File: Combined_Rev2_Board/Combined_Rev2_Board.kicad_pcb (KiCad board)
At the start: 4 copper layers, 121.9 x 106.8 mm, 178 parts, among them CN1 Conn_02x19_Odd_Even, CN1 USB_C_Receptacle_PowerOnly_6P, CN2 B2B-XH-A, CN2 Conn_02x19_Odd_Even, CN3 522070860, CN3 Molex FPC 541044031, CN4 Conn_01x02_Pin, CN4 Molex FPC 52271-0679, CN5 Conn_01x02_Pin, CN5 Conn_02x20_Odd_Even, CN6 Conn_01x02_Pin, CN7 Conn_01x02_Pin, J1 522070860, J1 Conn_01x02_Pin, J1 MIllMaxSpringConnector, J2 MIllMaxSpringConnector, J3 MIllMaxSpringConnector, J4 MIllMaxSpringConnector, J5 Conn_01x02_Pin, J5 MIllMaxSpringConnector, J6 Conn_01x02_Pin, J6 MIllMaxSpringConnector, J7 Conn_01x02_Pin, J7 MIllMaxSpringConnector, J8 MIllMaxSpringConnector, Q1 SI2347DS-TI-GE3CT, Q3 DMG3406L-7, Q4 SSM3J358R, SW2 Rocker Switch SPST, U1 AP5725WG-7, U10 LTC6252, U11 ADA4807-1, U11 MCP73831-2-OT, U12 LTC6252, U13 ADA4807-1, U14 LTC6252, U15 ADA4807-1, U16 LTC6252, U17 ADA4807-1, U2 ADA4807-2ACP, U2 LD39200, U3 ADR4530, U4 ADA4807-2ACP, U5 ADP7118-1.8, U6 ADA4807-2ACP, U7 AD4002_LFSCP-10, U8 AD4002_LFSCP-10, U8 TPS2400, U9 LD39200_Fixed

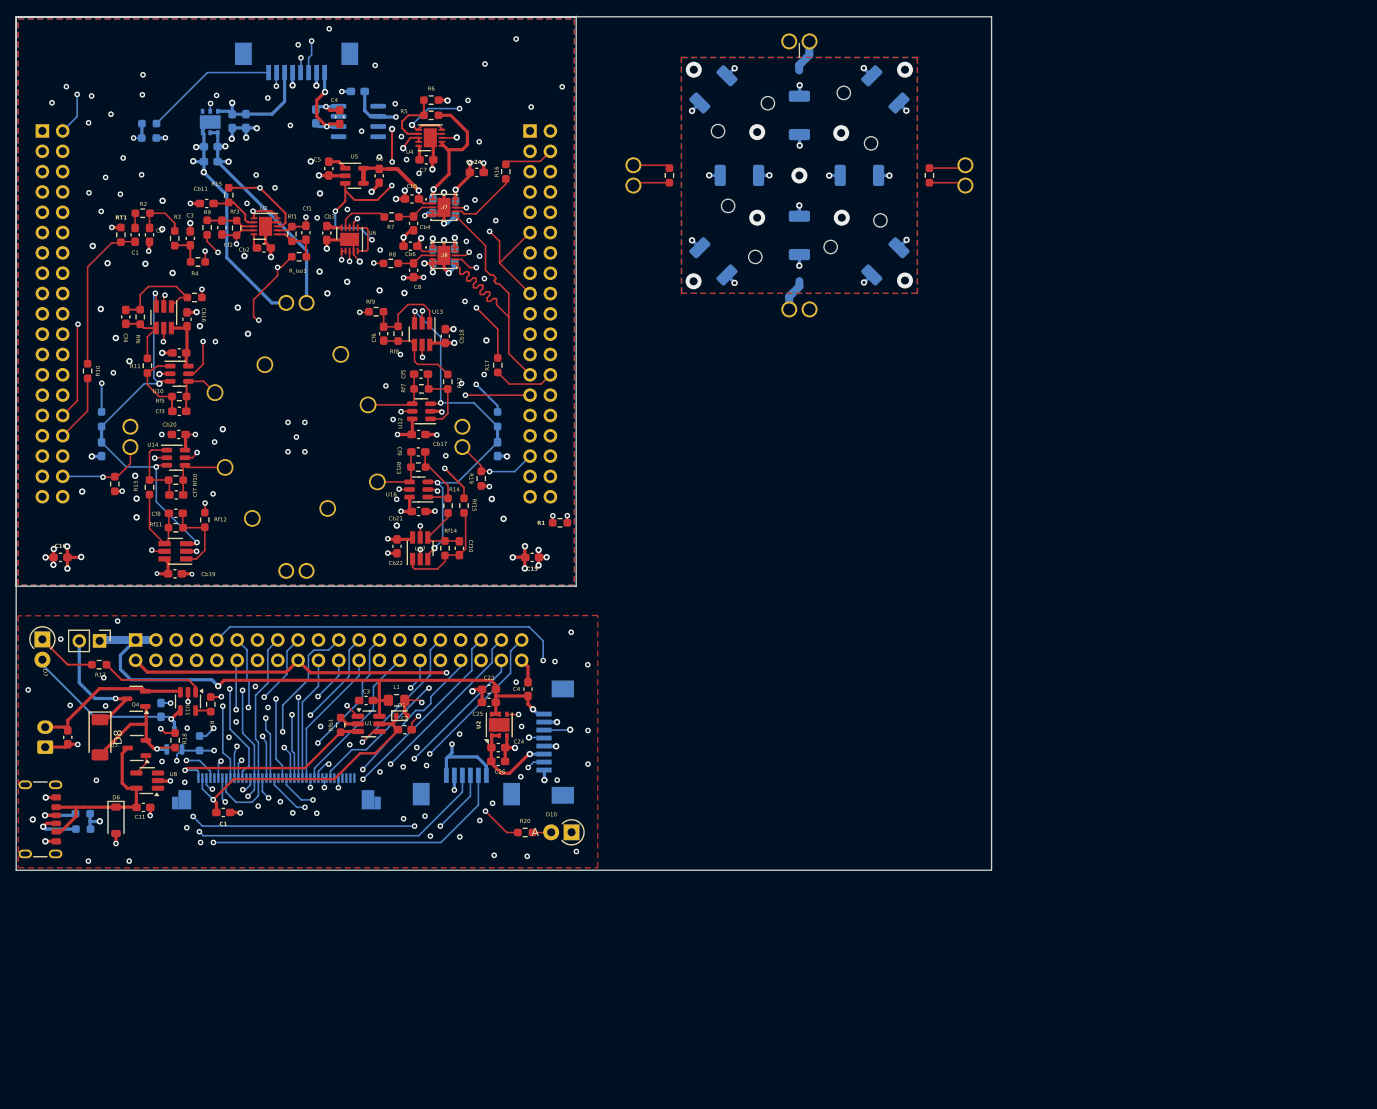
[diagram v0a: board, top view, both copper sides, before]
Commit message: Final commit before order
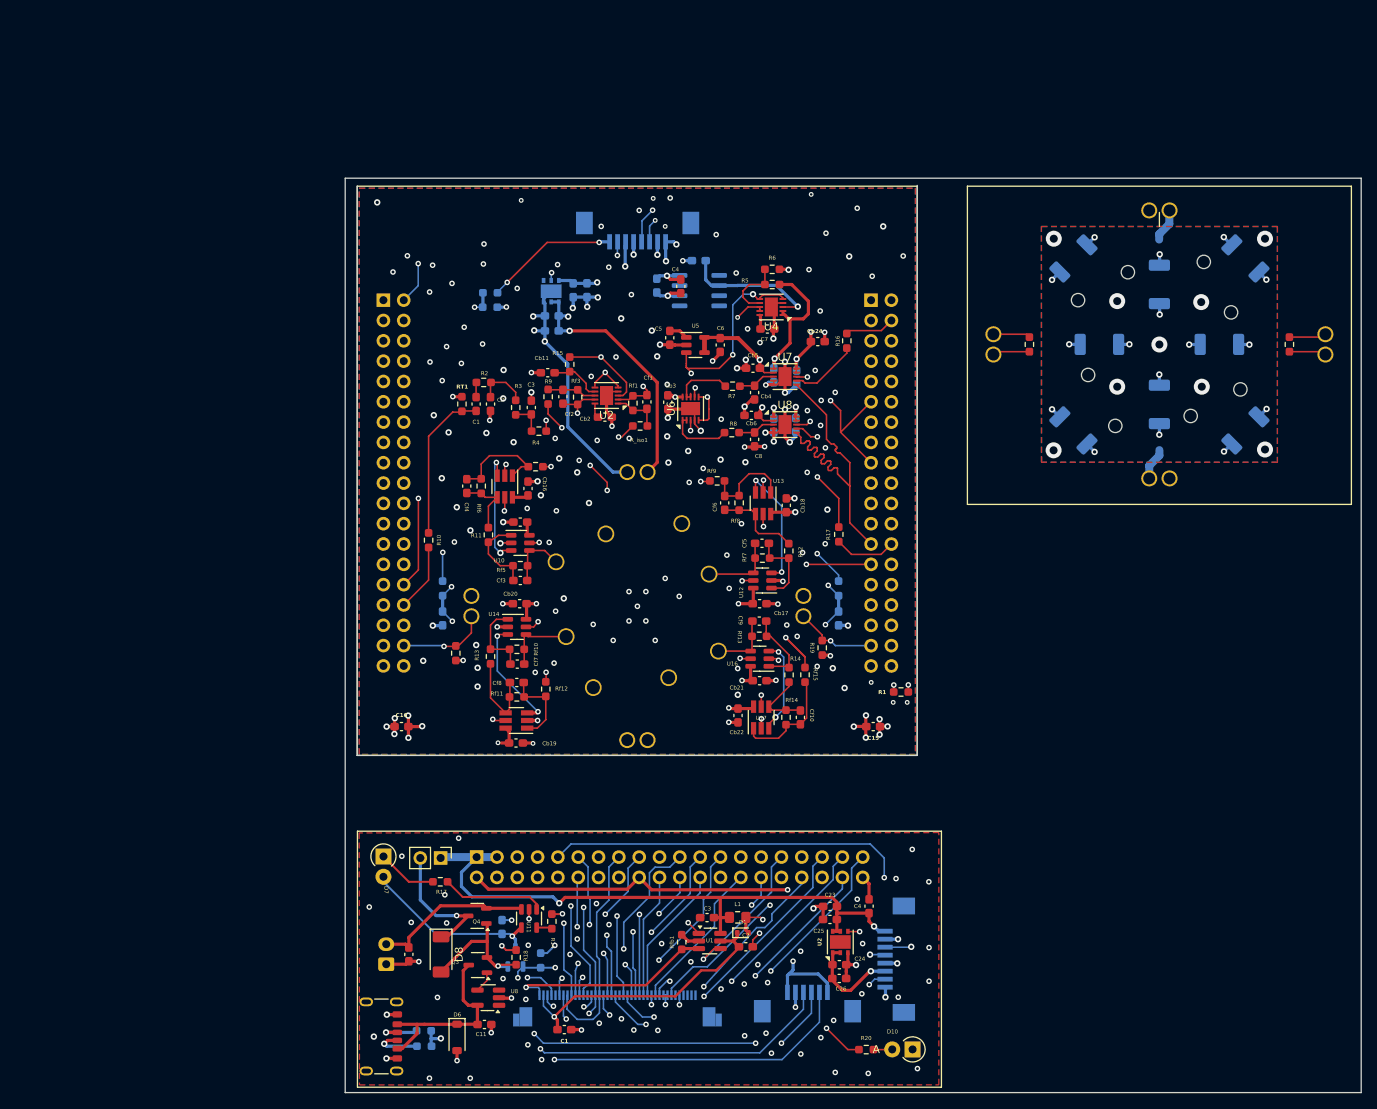
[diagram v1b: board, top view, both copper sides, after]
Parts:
- removed the C1 at (32.8, 109.3)
- removed the C1 at (21.7, 37.1)
- removed the C11 at (22.8, 108.7)
- removed the C11 at (49.6, 19.2)
- removed the C2 at (23.5, 37.1)
- removed the C2 at (55.5, 98.9)
- removed the C3 at (28.6, 37.5)
- removed the C3 at (50.6, 95.3)
- removed the C4 at (47.3, 22.4)
- removed the C4 at (70.9, 93.9)
- removed the CN1 at (8.80, 110.1)
- removed the CN1 at (10.2, 24.1)
- removed the CN2 at (71.1, 24.1)
- removed the CN2 at (10.5, 101.1)
- removed the CN3 at (39.4, 107.5)
- removed the CN3 at (41.9, 13.7)
- removed the CN4 at (21.1, 62.3)
- removed the CN4 at (63.2, 108.1)
- removed the CN5 at (62.6, 62.3)
- removed the CN5 at (21.8, 87.7)
- removed the J1 at (51.9, 66.6)
- removed the J1 at (104.8, 12.9)
- removed the J1 at (76.0, 100.5)
- removed the J5 at (51.5, 57.0)
- removed the J5 at (104.8, 46.4)
- removed the J6 at (84.0, 29.6)
- removed the J6 at (32.7, 55.0)
- removed the J7 at (47.5, 52.0)
- removed the J7 at (125.5, 29.6)
- removed the R1 at (74.8, 73.1)
- removed the R1 at (15.2, 109.4)
- removed the R10 at (15.8, 54.1)
- removed the R10 at (104.8, 22.1)
- removed the R11 at (23.3, 53.4)
- removed the R11 at (94.0, 18.9)
- removed the R12 at (60.8, 55.4)
- removed the R12 at (97.3, 29.6)
- removed the R13 at (23.5, 68.6)
- removed the R13 at (112.3, 29.6)
- removed the R14 at (60.9, 70.9)
- removed the R14 at (31.2, 95.8)
- removed the R14 at (104.8, 37.1)
- removed the R15 at (33.4, 32.1)
- removed the R15 at (94.0, 40.4)
- removed the R16 at (68.1, 29.2)
- removed the R16 at (115.5, 40.4)
- removed the R17 at (67.1, 53.4)
- removed the R17 at (17.3, 90.8)
- removed the R18 at (19.2, 68.2)
- removed the R18 at (26.7, 100.3)
- removed the R2 at (22.7, 34.4)
- removed the R2 at (15.3, 111.4)
- removed the R20 at (70.5, 111.8)
- removed the R20 at (23.5, 23.2)
- removed the R9 at (30.7, 36.2)
- removed the R9 at (115.5, 18.9)
- removed the U11 at (25.3, 47.4)
- removed the U11 at (28.4, 95.4)
- removed the U2 at (67.3, 98.3)
- removed the U2 at (38.0, 36.0)
- removed the U8 at (23.3, 105.3)
- removed the U8 at (60.4, 39.6)
- added C1: 1uF, Capacitor_SMD:C_0603_1608Metric_Pad1.08x0.95mm_HandSolder, F.Cu at (75.4, 136.4)
- added C1: 100p, Capacitor_SMD:C_0603_1608Metric_Pad1.08x0.95mm_HandSolder, F.Cu at (64.4, 58.2)
- added C11: 0.1u, Capacitor_SMD:C_0603_1608Metric_Pad1.08x0.95mm_HandSolder, F.Cu at (65.4, 135.8)
- added C11: 1uF, Capacitor_SMD:C_0603_1608Metric_Pad1.08x0.95mm_HandSolder, B.Cu at (92.2, 40.3)
- added C2: 1uF, Capacitor_SMD:C_0603_1608Metric_Pad1.08x0.95mm_HandSolder, F.Cu at (98.1, 126.1)
- added C2: 47p, Capacitor_SMD:C_0603_1608Metric_Pad1.08x0.95mm_HandSolder, F.Cu at (66.2, 58.2)
- added C3: 1uF, Capacitor_SMD:C_0603_1608Metric_Pad1.08x0.95mm_HandSolder, F.Cu at (93.2, 122.4)
- added C3: 47p, Capacitor_SMD:C_0603_1608Metric_Pad1.08x0.95mm_HandSolder, F.Cu at (71.3, 58.7)
- added C4: 1uF, Capacitor_SMD:C_0603_1608Metric_Pad1.08x0.95mm_HandSolder, F.Cu at (90.0, 43.5)
- added C4: 22u, Capacitor_SMD:C_0603_1608Metric_Pad1.08x0.95mm_HandSolder, F.Cu at (113.5, 121.0)
- added CN1: USB_C_Receptacle_PowerOnly_6P, Connector_USB:USB_C_Receptacle_GCT_USB4125-xx-x_6P_TopMnt_Horizontal, F.Cu at (51.4, 137.3)
- added CN1: Conn_02x19_Odd_Even, Connector_PinSocket_2.54mm:PinSocket_2x19_P2.54mm_Vertical, B.Cu at (52.8, 45.2)
- added CN2: Conn_02x19_Odd_Even, Connector_PinSocket_2.54mm:PinSocket_2x19_P2.54mm_Vertical, B.Cu at (113.7, 45.2)
- added CN2: B2B-XH-A, Connector_JST:JST_XH_B2B-XH-A_1x02_P2.50mm_Vertical, B.Cu at (53.1, 128.2)
- added CN3: 522070860, GenIILibrary:CON_522070860_MOL, B.Cu at (84.5, 34.8)
- added CN3: Molex FPC 541044031, GenIILibrary:CON_541044031_MOL, B.Cu at (82.0, 134.6)
- added CN4: Conn_01x02_Pin, GenIILibrary:Samtec_Pin_Socket_SS_102_G_2, F.Cu at (63.8, 83.5)
- added CN4: Molex FPC 52271-0679, GenIILibrary:MOLEX_52271-0679, B.Cu at (105.8, 135.3)
- added CN5: Conn_01x02_Pin, GenIILibrary:Samtec_Pin_Socket_SS_102_G_2, F.Cu at (105.3, 83.5)
- added CN5: Conn_02x20_Odd_Even, Connector_PinHeader_2.54mm:PinHeader_2x20_P2.54mm_Vertical, B.Cu at (64.4, 114.9)
- added J1: MIllMaxSpringConnector, TCGenI_Rev3_Redo:MillMax_0914-2, F.Cu at (94.5, 87.8)
- added J1: Conn_01x02_Pin, GenIILibrary:Samtec_Pin_Socket_SS_102_G_2, F.Cu at (149.8, 34.0)
- added J1: 522070860, GenIILibrary:CON_522070860_MOL, B.Cu at (118.6, 127.6)
- added J5: MIllMaxSpringConnector, TCGenI_Rev3_Redo:MillMax_0914-2, F.Cu at (94.1, 78.1)
- added J5: Conn_01x02_Pin, GenIILibrary:Samtec_Pin_Socket_SS_102_G_2, F.Cu at (149.8, 67.5)
- added J6: Conn_01x02_Pin, GenIILibrary:Samtec_Pin_Socket_SS_102_G_2, F.Cu at (129.0, 50.8)
- added J6: MIllMaxSpringConnector, TCGenI_Rev3_Redo:MillMax_0914-2, F.Cu at (75.3, 76.1)
- added J7: MIllMaxSpringConnector, TCGenI_Rev3_Redo:MillMax_0914-2, F.Cu at (90.1, 73.2)
- added J7: Conn_01x02_Pin, GenIILibrary:Samtec_Pin_Socket_SS_102_G_2, F.Cu at (170.5, 50.8)
- added R1: 33, Resistor_SMD:R_0603_1608Metric_Pad0.98x0.95mm_HandSolder, F.Cu at (117.5, 94.2)
- added R1: 5.1k, Resistor_SMD:R_0603_1608Metric_Pad0.98x0.95mm_HandSolder, B.Cu at (57.8, 136.6)
- added R10: 33, Resistor_SMD:R_0603_1608Metric_Pad0.98x0.95mm_HandSolder, F.Cu at (58.4, 75.2)
- added R10: 50, Resistor_SMD:R_2010_5025Metric_Pad1.40x2.65mm_HandSolder, B.Cu at (149.8, 43.3)
- added R11: 1k, Resistor_SMD:R_0603_1608Metric_Pad0.98x0.95mm_HandSolder, F.Cu at (65.9, 74.6)
- added R11: 50, Resistor_SMD:R_2010_5025Metric_Pad1.40x2.65mm_HandSolder, B.Cu at (139.0, 40.0)
- added R12: 1k, Resistor_SMD:R_0603_1608Metric_Pad0.98x0.95mm_HandSolder, F.Cu at (103.5, 76.6)
- added R12: 50, Resistor_SMD:R_2010_5025Metric_Pad1.40x2.65mm_HandSolder, B.Cu at (142.3, 50.8)
- added R13: 1k, Resistor_SMD:R_0603_1608Metric_Pad0.98x0.95mm_HandSolder, F.Cu at (66.2, 89.8)
- added R13: 50, Resistor_SMD:R_2010_5025Metric_Pad1.40x2.65mm_HandSolder, B.Cu at (157.3, 50.8)
- added R14: 1k, Resistor_SMD:R_0603_1608Metric_Pad0.98x0.95mm_HandSolder, F.Cu at (103.5, 92.1)
- added R14: 2k, Resistor_SMD:R_0603_1608Metric_Pad0.98x0.95mm_HandSolder, F.Cu at (73.8, 122.9)
- added R14: 50, Resistor_SMD:R_2010_5025Metric_Pad1.40x2.65mm_HandSolder, B.Cu at (149.8, 58.3)
- added R15: 1k, Resistor_SMD:R_0603_1608Metric_Pad0.98x0.95mm_HandSolder, F.Cu at (76.1, 53.3)
- added R15: 50, Resistor_SMD:R_2010_5025Metric_Pad1.40x2.65mm_HandSolder, B.Cu at (139.0, 61.5)
- added R16: 33, Resistor_SMD:R_0603_1608Metric_Pad0.98x0.95mm_HandSolder, F.Cu at (110.7, 50.3)
- added R16: 50, Resistor_SMD:R_2010_5025Metric_Pad1.40x2.65mm_HandSolder, B.Cu at (160.5, 61.5)
- added R17: 1k, Resistor_SMD:R_0603_1608Metric_Pad0.98x0.95mm_HandSolder, F.Cu at (59.9, 118.0)
- added R17: 33, Resistor_SMD:R_0603_1608Metric_Pad0.98x0.95mm_HandSolder, F.Cu at (109.7, 74.5)
- added R18: 1k, Resistor_SMD:R_0603_1608Metric_Pad0.98x0.95mm_HandSolder, F.Cu at (61.8, 89.4)
- added R18: 10k, Resistor_SMD:R_0603_1608Metric_Pad0.98x0.95mm_HandSolder, F.Cu at (69.4, 127.4)
- added R2: 10k, Resistor_SMD:R_0603_1608Metric_Pad0.98x0.95mm_HandSolder, F.Cu at (65.3, 55.5)
- added R2: 5.1k, Resistor_SMD:R_0603_1608Metric_Pad0.98x0.95mm_HandSolder, B.Cu at (57.9, 138.5)
- added R20: 1k, Resistor_SMD:R_0603_1608Metric_Pad0.98x0.95mm_HandSolder, F.Cu at (113.1, 138.9)
- added R20: 10k, Resistor_SMD:R_0603_1608Metric_Pad0.98x0.95mm_HandSolder, B.Cu at (66.1, 44.3)
- added R9: 1k, Resistor_SMD:R_0603_1608Metric_Pad0.98x0.95mm_HandSolder, F.Cu at (73.4, 57.3)
- added R9: 50, Resistor_SMD:R_2010_5025Metric_Pad1.40x2.65mm_HandSolder, B.Cu at (160.5, 40.0)
- added U11: MCP73831-2-OT, Package_TO_SOT_SMD:SOT-23-5, F.Cu at (71.0, 122.5)
- added U11: ADA4807-1, Package_TO_SOT_SMD:SOT-23-6_Handsoldering, F.Cu at (68.0, 68.5)
- added U2: LD39200, Package_DFN_QFN:DFN-6-1EP_3x3mm_P0.95mm_EP1.7x2.6mm, F.Cu at (109.9, 125.5)
- added U2: ADA4807-2ACP, CustomPaste:LFCSP-WD-10-1EP_3x3mm_P0.5mm_EP1.64x2.38mm, F.Cu at (80.7, 57.2)
- added U8: TPS2400, Package_TO_SOT_SMD:SOT-23-5_HandSoldering, F.Cu at (65.9, 132.4)
- added U8: AD4002_LFSCP-10, Package_CSP:LFCSP-WD-10-1EP_3x3mm_P0.5mm_EP1.64x2.38mm, F.Cu at (103.0, 60.8)
- RT1: value 0 -> NC
- U4, U6: footprint Package_CSP:LFCSP-WD-10-1EP_3x3mm_P0.5mm_EP1.64x2.38mm -> CustomPaste:LFCSP-WD-10-1EP_3x3mm_P0.5mm_EP1.64x2.38mm
- U7: footprint footprints:CP_10_9_ADI -> Package_CSP:LFCSP-WD-10-1EP_3x3mm_P0.5mm_EP1.64x2.38mm
- moved C20 50.5 mm to (56.0, 127.0)
- moved C23 50.5 mm to (108.6, 121.0)
- moved C25 50.5 mm to (108.6, 122.7)
- moved D1 50.5 mm to (97.7, 124.3)
- moved D10 50.5 mm to (118.9, 138.9)
- moved D6 50.5 mm to (62.0, 137.4)
- moved D8 50.5 mm to (60.0, 127.0)
- moved Q1 50.5 mm to (69.3, 127.4)
- moved Q3 50.5 mm to (64.6, 128.4)
- moved RPU1 50.5 mm to (72.4, 127.8)
- moved Rfb1 50.5 mm to (90.1, 125.5)
- moved C19 50.5 mm to (67.6, 123.6)
- moved D7 50.5 mm to (52.8, 114.8)
- moved L1 50.5 mm to (97.1, 122.4)
- moved Q4 50.5 mm to (64.5, 122.2)
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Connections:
- C10 pad 1: (no net) -> GND
- C10 pad 2: (no net) -> Vdd_Main
- C12 pad 1: (no net) -> /Heater_Interface/Heater+
- C12 pad 2: (no net) -> GND
- C13 pad 1: (no net) -> Vcc
- C13 pad 2: (no net) -> GND
- C14 pad 1: (no net) -> /Heater_Interface/Heater+
- C14 pad 2: (no net) -> GND
- C15 pad 1: (no net) -> GND
- C15 pad 2: (no net) -> Vdd_Main
- C16 pad 1: (no net) -> GND
- C16 pad 2: (no net) -> Vdd_Main
- C19 pad 1: (no net) -> GND
- C19 pad 2: (no net) -> Net-(D7-A)
- C20 pad 1: (no net) -> /V_Batt
- C20 pad 2: (no net) -> GND
- C23 pad 1: (no net) -> GND
- C23 pad 2: (no net) -> /Vcc
- C24 pad 1: (no net) -> /3V3_Main
- C24 pad 2: (no net) -> GND
- C25 pad 1: (no net) -> /Vcc
- C25 pad 2: (no net) -> GND
- C26 pad 1: (no net) -> /3V3_Main
- C26 pad 2: (no net) -> GND
- C5 pad 1: (no net) -> Vdd_Main
- C5 pad 2: (no net) -> GND
- C6 pad 1: (no net) -> Vdd_ADC
- C6 pad 2: (no net) -> GND
- C7 pad 1: (no net) -> Vdd_Main
- C7 pad 2: (no net) -> GND
- C8 pad 1: (no net) -> GND
- C8 pad 2: (no net) -> Net-(U8-IN+)
- C9 pad 1: (no net) -> GND
- C9 pad 2: (no net) -> Vcc
- CN6 pad 1: (no net) -> unconnected-(CN6-Pin_1-Pad1)
- CN6 pad 2: (no net) -> unconnected-(CN6-Pin_2-Pad2)
- CN7 pad 1: (no net) -> GND
- CN7 pad 2: (no net) -> /Heater_Interface/Heater+
- Cb1 pad 1: (no net) -> GND
- Cb1 pad 2: (no net) -> /ABBCore_Alt/TIA_2/V_MID
- Cb10 pad 1: (no net) -> GND
- Cb10 pad 2: (no net) -> Vdd_Main
- Cb11 pad 1: (no net) -> GND
- Cb11 pad 2: (no net) -> Net-(U2B-+)
- Cb12 pad 1: (no net) -> GND
- Cb12 pad 2: (no net) -> /ABBCore_Alt/TIA_1/V_MID
- Cb15 pad 1: (no net) -> GND
- Cb15 pad 2: (no net) -> Vdd_Main
- Cb16 pad 1: (no net) -> GND
- Cb16 pad 2: (no net) -> Vdd_Main
- Cb17 pad 1: (no net) -> GND
- Cb17 pad 2: (no net) -> Vdd_Main
- Cb18 pad 1: (no net) -> GND
- Cb18 pad 2: (no net) -> Vdd_Main
- Cb19 pad 1: (no net) -> GND
- Cb19 pad 2: (no net) -> Vdd_Main
- Cb2 pad 1: (no net) -> GND
- Cb2 pad 2: (no net) -> Vdd_Main
- Cb20 pad 1: (no net) -> GND
- Cb20 pad 2: (no net) -> Vdd_Main
- Cb21 pad 1: (no net) -> GND
- Cb21 pad 2: (no net) -> Vdd_Main
- Cb22 pad 1: (no net) -> GND
- Cb22 pad 2: (no net) -> Vdd_Main
- Cb24 pad 1: (no net) -> GND
- Cb24 pad 2: (no net) -> Vdd_Main
- Cb3 pad 1: (no net) -> Vdd_Main
- Cb3 pad 2: (no net) -> GND
- Cb4 pad 1: (no net) -> GND
- Cb4 pad 2: (no net) -> Net-(U7-IN+)
- Cb5 pad 1: (no net) -> Vdd_ADC
- Cb5 pad 2: (no net) -> GND
- Cb6 pad 1: (no net) -> Vdd_ADC
- Cb6 pad 2: (no net) -> GND
- Cb7 pad 1: (no net) -> GND
- Cb7 pad 2: (no net) -> ADC_VREF
- Cb8 pad 1: (no net) -> GND
- Cb8 pad 2: (no net) -> ADC_VREF
- Cb9 pad 1: (no net) -> GND
- Cb9 pad 2: (no net) -> Vdd_Main
- Cf1 pad 1: (no net) -> Net-(Cf1-Pad1)
- Cf1 pad 2: (no net) -> Net-(U2A--)
- Cf10 pad 1: (no net) -> Net-(U17--)
- Cf10 pad 2: (no net) -> Net-(Cf10-Pad2)
- Cf2 pad 1: (no net) -> Net-(U2B--)
- Cf2 pad 2: (no net) -> /ABBCore_Alt/V_Exc
- Cf3 pad 1: (no net) -> CCOut_1
- Cf3 pad 2: (no net) -> Net-(Cf3-Pad2)
- Cf4 pad 1: (no net) -> Net-(U11--)
- Cf4 pad 2: (no net) -> Net-(Cf4-Pad2)
- Cf5 pad 1: (no net) -> CCOut_2
- Cf5 pad 2: (no net) -> Net-(Cf5-Pad2)
- Cf6 pad 1: (no net) -> Net-(U13--)
- Cf6 pad 2: (no net) -> Net-(Cf6-Pad2)
- Cf7 pad 1: (no net) -> CCOut_3
- Cf7 pad 2: (no net) -> Net-(Cf7-Pad2)
- Cf8 pad 1: (no net) -> Net-(U15--)
- Cf8 pad 2: (no net) -> Net-(Cf8-Pad2)
- Cf9 pad 1: (no net) -> CCOut_4
- Cf9 pad 2: (no net) -> Net-(Cf9-Pad2)
- D1 pad 1: (no net) -> /LED+
- D1 pad 2: (no net) -> Net-(D1-A)
- D10 pad 1: (no net) -> GND
- D10 pad 2: (no net) -> Net-(D10-A)
- D6 pad 1: (no net) -> /Power_Management_Minimal/VBus
- D6 pad 2: (no net) -> GND
- D7 pad 1: (no net) -> Net-(D7-K)
- D7 pad 2: (no net) -> Net-(D7-A)
- D8 pad 1: (no net) -> Net-(D8-K)
- D8 pad 2: (no net) -> /Power_Management_Minimal/5V_USB
- J2 pad 1: (no net) -> CCOut_3
- J3 pad 1: (no net) -> /ABBCore_Alt/V_Drive
- J4 pad 1: (no net) -> /ABBCore_Alt/V_Drive
- J8 pad 1: (no net) -> /ABBCore_Alt/V_Drive
- L1 pad 1: (no net) -> /Vcc
- L1 pad 2: (no net) -> Net-(D1-A)
- Q1 pad 1: (no net) -> /~{CHARGE_EN}
- Q1 pad 2: (no net) -> /Power_Management_Minimal/5V_USB
- Q1 pad 3: (no net) -> Net-(D7-A)
- Q3 pad 1: (no net) -> Net-(Q3-G)
- Q3 pad 2: (no net) -> /Power_Management_Minimal/5V_USB
- Q3 pad 3: (no net) -> /Power_Management_Minimal/VBus
- Q4 pad 1: (no net) -> /Power_Management_Minimal/5V_USB
- Q4 pad 2: (no net) -> /V_Batt
- Q4 pad 3: (no net) -> Net-(D8-K)
- R19 pad 1: (no net) -> GND
- R19 pad 2: (no net) -> Vth_2
- R21 pad 1: (no net) -> /MCU Connections/PC1
- R21 pad 2: (no net) -> GND
- R3 pad 1: (no net) -> Net-(C2-Pad1)
- R3 pad 2: (no net) -> Net-(C3-Pad1)
- R4 pad 1: (no net) -> Net-(C3-Pad1)
- R4 pad 2: (no net) -> Net-(U2A--)
- R5 pad 1: (no net) -> ADC_VREF
- R5 pad 2: (no net) -> Net-(U4B-+)
- R6 pad 1: (no net) -> Net-(U4B-+)
- R6 pad 2: (no net) -> GND
- R7 pad 1: (no net) -> Net-(U7-IN+)
- R7 pad 2: (no net) -> Net-(U6B--)
- R8 pad 1: (no net) -> Net-(U8-IN+)
- R8 pad 2: (no net) -> Net-(U6A--)
- RPU1 pad 1: (no net) -> /~{CHARGE_EN}
- RPU1 pad 2: (no net) -> GND
- RT1 pad 1: (no net) -> GND
- RT1 pad 2: (no net) -> V_SIG
- R_iso1 pad 1: (no net) -> Net-(Cf1-Pad1)
- R_iso1 pad 2: (no net) -> /ABBCore_Alt/V_Drive
- Rf1 pad 1: (no net) -> Net-(Cf1-Pad1)
- Rf1 pad 2: (no net) -> Net-(U2A--)
- Rf10 pad 1: (no net) -> CCOut_3
- Rf10 pad 2: (no net) -> Net-(Cf7-Pad2)
- Rf11 pad 1: (no net) -> Net-(U15--)
- Rf11 pad 2: (no net) -> Net-(Cf8-Pad2)
- Rf12 pad 1: (no net) -> Net-(Cf8-Pad2)
- Rf12 pad 2: (no net) -> /ABBCore_Alt/V_Resp
- Rf13 pad 1: (no net) -> CCOut_4
- Rf13 pad 2: (no net) -> Net-(Cf9-Pad2)
- Rf14 pad 1: (no net) -> Net-(U17--)
- Rf14 pad 2: (no net) -> Net-(Cf10-Pad2)
- Rf15 pad 1: (no net) -> Net-(Cf10-Pad2)
- Rf15 pad 2: (no net) -> /ABBCore_Alt/V_Resp
- Rf16 pad 1: (no net) -> V_MID
- Rf16 pad 2: (no net) -> /ABBCore_Alt/TIA_2/V_MID
- Rf3 pad 1: (no net) -> Net-(U2B--)
- Rf3 pad 2: (no net) -> /ABBCore_Alt/V_Exc
- Rf4 pad 1: (no net) -> V_MID
- Rf4 pad 2: (no net) -> /ABBCore_Alt/TIA_1/V_MID
- Rf5 pad 1: (no net) -> CCOut_1
- Rf5 pad 2: (no net) -> Net-(Cf3-Pad2)
- Rf6 pad 1: (no net) -> Net-(U11--)
- Rf6 pad 2: (no net) -> Net-(Cf4-Pad2)
- Rf7 pad 1: (no net) -> CCOut_2
- Rf7 pad 2: (no net) -> Net-(Cf5-Pad2)
- Rf8 pad 1: (no net) -> Net-(U13--)
- Rf8 pad 2: (no net) -> Net-(Cf6-Pad2)
- Rf9 pad 1: (no net) -> Net-(Cf6-Pad2)
- Rf9 pad 2: (no net) -> /ABBCore_Alt/V_Resp
- Rfb1 pad 1: (no net) -> GND
- Rfb1 pad 2: (no net) -> /LED-
- Riso1 pad 1: (no net) -> Net-(Cf4-Pad2)
- Riso1 pad 2: (no net) -> /ABBCore_Alt/V_Resp
- SW2 pad 1: (no net) -> /Vcc
- SW2 pad 2: (no net) -> Net-(D8-K)
- TH5 pad 1: (no net) -> Net-(J7-Pin_1)
- TH5 pad 2: (no net) -> Net-(J7-Pin_2)
- TH7 pad 1: (no net) -> Net-(J6-Pin_1)
- TH7 pad 2: (no net) -> Net-(J6-Pin_2)
- U1 pad 1: (no net) -> Net-(D1-A)
- U1 pad 2: (no net) -> GND
- U1 pad 3: (no net) -> /LED-
- U1 pad 4: (no net) -> /PWM_EN
- U1 pad 5: (no net) -> /LED+
- U1 pad 6: (no net) -> /Vcc
- U10 pad 1: (no net) -> Net-(Cf3-Pad2)
- U10 pad 2: (no net) -> GND
- U10 pad 3: (no net) -> /ABBCore_Alt/TIA_1/V_MID
- U10 pad 4: (no net) -> CCOut_1
- U10 pad 5: (no net) -> ~{TIA1_SHDN}
- U10 pad 6: (no net) -> Vdd_Main
- U12 pad 1: (no net) -> Net-(Cf5-Pad2)
- U12 pad 2: (no net) -> GND
- U12 pad 3: (no net) -> /ABBCore_Alt/TIA_2/V_MID
- U12 pad 4: (no net) -> CCOut_2
- U12 pad 5: (no net) -> ~{TIA2_SHDN}
- U12 pad 6: (no net) -> Vdd_Main
- U13 pad 1: (no net) -> Net-(Cf6-Pad2)
- U13 pad 2: (no net) -> GND
- U13 pad 3: (no net) -> /ABBCore_Alt/TIA_2/V_MID
- U13 pad 4: (no net) -> Net-(U13--)
- U13 pad 5: (no net) -> ~{TIA2_SHDN}
- U13 pad 6: (no net) -> Vdd_Main
- U14 pad 1: (no net) -> Net-(Cf7-Pad2)
- U14 pad 2: (no net) -> GND
- U14 pad 3: (no net) -> /ABBCore_Alt/TIA_1/V_MID
- U14 pad 4: (no net) -> CCOut_3
- U14 pad 5: (no net) -> ~{TIA3_SHDN}
- U14 pad 6: (no net) -> Vdd_Main
- U15 pad 1: (no net) -> Net-(Cf8-Pad2)
- U15 pad 2: (no net) -> GND
- U15 pad 3: (no net) -> /ABBCore_Alt/TIA_1/V_MID
- U15 pad 4: (no net) -> Net-(U15--)
- U15 pad 5: (no net) -> ~{TIA3_SHDN}
- U15 pad 6: (no net) -> Vdd_Main
- U16 pad 1: (no net) -> Net-(Cf9-Pad2)
- U16 pad 2: (no net) -> GND
- U16 pad 3: (no net) -> /ABBCore_Alt/TIA_2/V_MID
- U16 pad 4: (no net) -> CCOut_4
- U16 pad 5: (no net) -> ~{TIA4_SHDN}
- U16 pad 6: (no net) -> Vdd_Main
- U17 pad 1: (no net) -> Net-(Cf10-Pad2)
- U17 pad 2: (no net) -> GND
- U17 pad 3: (no net) -> /ABBCore_Alt/TIA_2/V_MID
- U17 pad 4: (no net) -> Net-(U17--)
- U17 pad 5: (no net) -> ~{TIA4_SHDN}
- U17 pad 6: (no net) -> Vdd_Main
- U3 pad 1: (no net) -> unconnected-(U3-NC-Pad1)
- U3 pad 2: (no net) -> Vdd_Main
- U3 pad 3: (no net) -> unconnected-(U3-NC-Pad3)
- U3 pad 4: (no net) -> GND
- U3 pad 5: (no net) -> unconnected-(U3-NC-Pad5)
- U3 pad 6: (no net) -> Net-(U3-OUT)
- U3 pad 7: (no net) -> unconnected-(U3-NC-Pad7)
- U3 pad 8: (no net) -> unconnected-(U3-NC-Pad8)
- U4 pad 1: (no net) -> ADC_VREF
- U4 pad 10: (no net) -> Vdd_Main
- U4 pad 11: (no net) -> GND
- U4 pad 2: (no net) -> ADC_VREF
- U4 pad 3: (no net) -> Net-(U3-OUT)
- U4 pad 4: (no net) -> GND
- U4 pad 5: (no net) -> ~{ADC1_SHDN}
- U4 pad 6: (no net) -> ~{ADC1_SHDN}
- U4 pad 7: (no net) -> Net-(U4B-+)
- U4 pad 8: (no net) -> V_MID
- U4 pad 9: (no net) -> V_MID
- U5 pad 1: (no net) -> Vdd_Main
- U5 pad 2: (no net) -> GND
- U5 pad 3: (no net) -> ~{ADC1_SHDN}
- U5 pad 4: (no net) -> Vdd_ADC
- U5 pad 5: (no net) -> Vdd_ADC
- U6 pad 1: (no net) -> Net-(U6A--)
- U6 pad 10: (no net) -> Vdd_Main
- U6 pad 11: (no net) -> GND
- U6 pad 2: (no net) -> Net-(U6A--)
- U6 pad 3: (no net) -> /ABBCore_Alt/V_Resp
- U6 pad 4: (no net) -> GND
- U6 pad 5: (no net) -> ~{ADC1_SHDN}
- U6 pad 6: (no net) -> ~{ADC1_SHDN}
- U6 pad 7: (no net) -> /ABBCore_Alt/V_Exc
- U6 pad 8: (no net) -> Net-(U6B--)
- U6 pad 9: (no net) -> Net-(U6B--)
- U7 pad 1: (no net) -> ADC_VREF
- U7 pad 10: (no net) -> Vdd_Main
- U7 pad 11: (no net) -> GND
- U7 pad 2: (no net) -> Vdd_ADC
- U7 pad 3: (no net) -> Net-(U7-IN+)
- U7 pad 4: (no net) -> GND
- U7 pad 5: (no net) -> GND
- U7 pad 6: (no net) -> CNV
- U7 pad 7: (no net) -> Dataout0
- U7 pad 8: (no net) -> MCU_SCK
- U7 pad 9: (no net) -> Vdd_Main
- U9 pad 1: (no net) -> /Heater_Interface/Heater+
- U9 pad 2: (no net) -> /Heater_Interface/Heater+
- U9 pad 3: (no net) -> GND
- U9 pad 4: (no net) -> unconnected-(U9-PWRGD-Pad4)
- U9 pad 5: (no net) -> Heater_EN
- U9 pad 6: (no net) -> Vcc
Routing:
- net (no net): track 3194.1 -> 0.00 mm, vias 394 -> 0
- net GND: track 0.00 -> 188.4 mm, vias 0 -> 188
- net V_MID: track 0.00 -> 118.4 mm, vias 0 -> 4
- net /V_Batt: track 0.00 -> 98.9 mm, vias 0 -> 1
- net /ABBCore_Alt/V_Resp: track 0.00 -> 94.0 mm, vias 0 -> 5
- net UART_TX: track 0.00 -> 91.9 mm, vias 0 -> 2
- net /ABBCore_Alt/V_Drive: track 0.00 -> 89.8 mm, vias 0 -> 5
- net /3V3_Pi: track 0.00 -> 81.2 mm, vias 0 -> 3
- net /Vcc: track 0.00 -> 78.4 mm, vias 0 -> 2
- net /~{CHARGE_EN}: track 0.00 -> 68.0 mm, vias 0 -> 3
- net Vdd_Main: track 0.00 -> 67.8 mm, vias 0 -> 75
- net ~{ADC1_SHDN}: track 0.00 -> 65.3 mm, vias 0 -> 5
- net /UART_TX: track 0.00 -> 62.5 mm, vias 0 -> 1
- net /~{INT}: track 0.00 -> 62.4 mm, vias 0 -> 1
- net /SDA: track 0.00 -> 60.8 mm, vias 0 -> 3
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- added copper zone on B.Cu, net GND
- added copper zone on F.Cu, net GND
- added copper zone on In1.Cu, net GND
- added copper zone on In2.Cu, net GND
- added copper zone on In1.Cu, net Net-(J1-Pin_2)
- added copper zone on In2.Cu, net Net-(J1-Pin_2)
- added copper zone on B.Cu, net Vdd_Heater_2
- added copper zone on F.Cu, net Vdd_Heater_2
- added copper zone on F.Cu, net Vdd_Main
- added copper zone on In2.Cu, net Vdd_Main
- removed copper zone on B.Cu, net (none)
- removed copper zone on F.Cu, net (none)
- removed copper zone on In1.Cu, net (none)
- removed copper zone on In2.Cu, net (none)
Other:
- board size 121.9 x 106.8 mm -> 127 x 114.3 mm
